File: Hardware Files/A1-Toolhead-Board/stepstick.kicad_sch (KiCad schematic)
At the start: 18 parts, among them J1 Motor_E, U1 TMC2209-LA

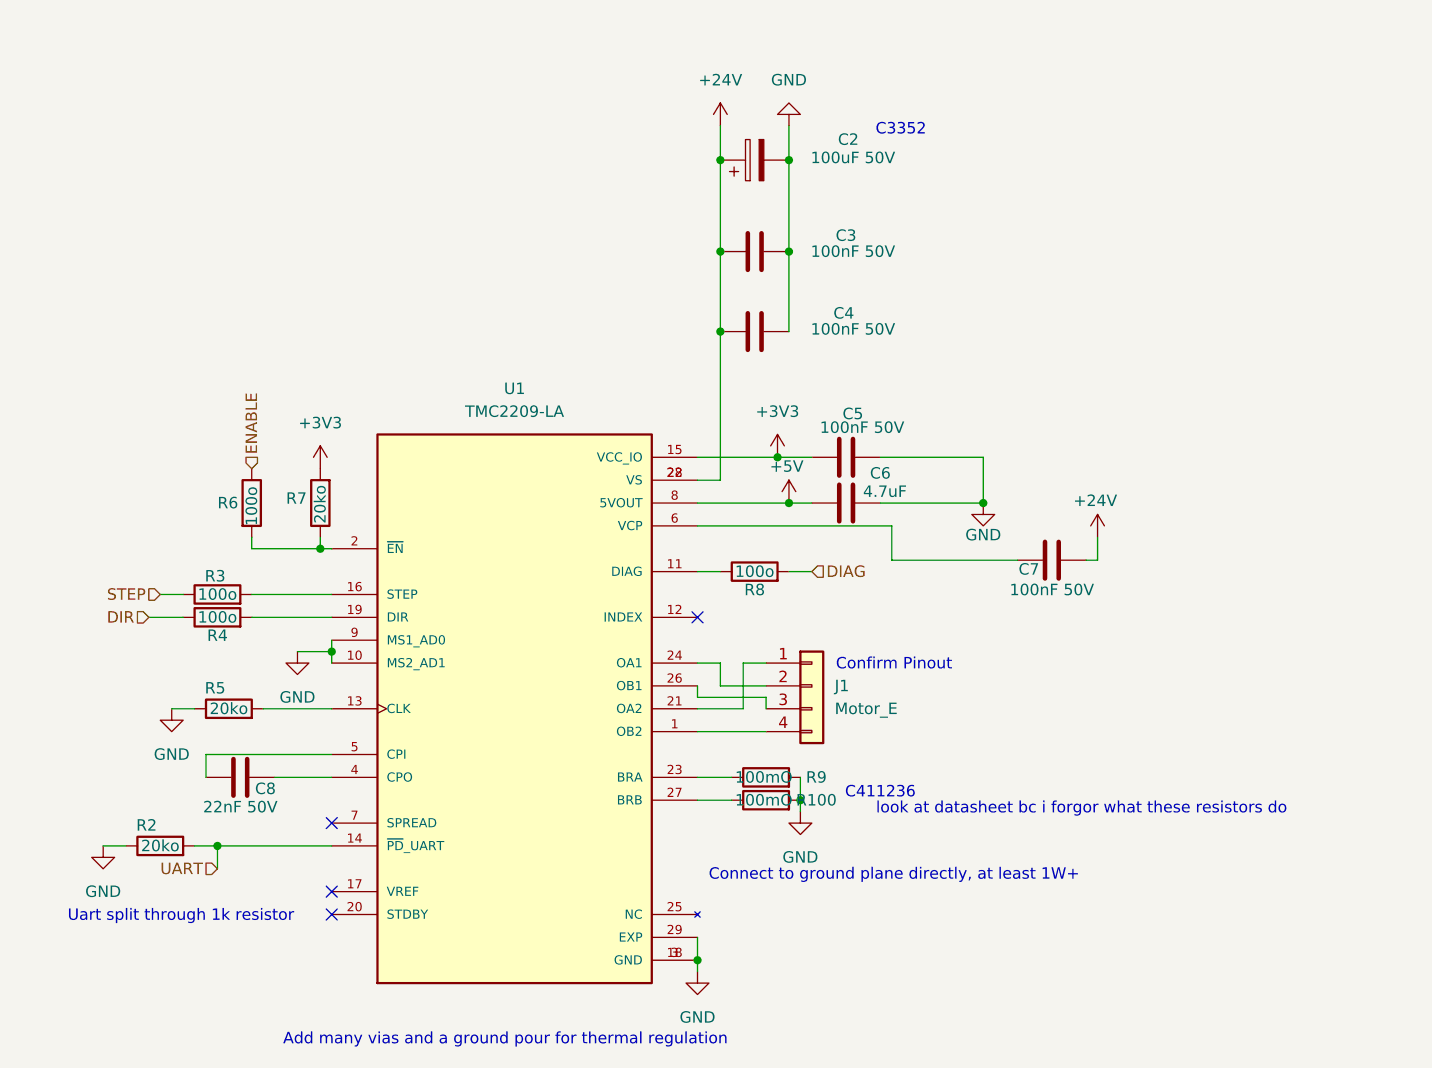
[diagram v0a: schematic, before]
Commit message: e
e
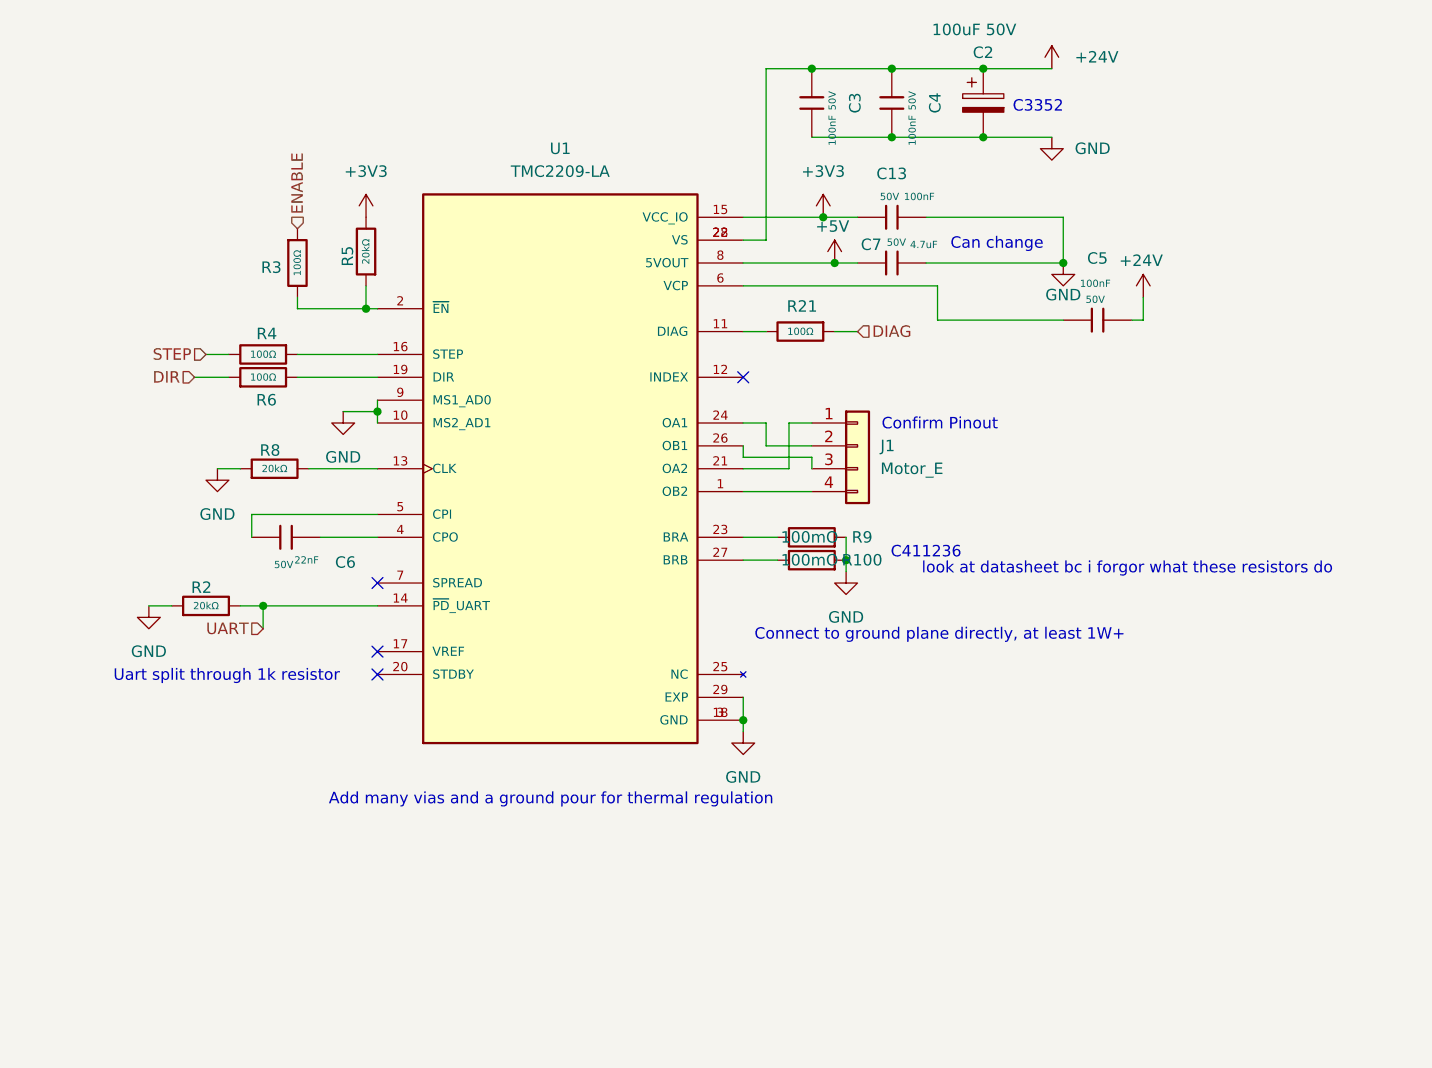
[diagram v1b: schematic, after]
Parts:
- removed C3, C4, C5, C7: 100nF 50V, Capacitor_SMD:C_0402_1005Metric, symbol Device:C
- removed C6: 4.7uF, Capacitor_SMD:C_0201_0603Metric, symbol Device:C
- removed C8: 22nF 50V, Capacitor_SMD:C_0402_1005Metric, symbol Device:C
- removed R2, R5, R7: 20ko, Resistor_SMD:R_0402_1005Metric, symbol Device:R
- removed R3, R4, R6, R8: 100o, Resistor_SMD:R_0402_1005Metric, symbol Device:R
- added C13, C3, C4, C5: 100nF, PCM_JLCPCB:C_0402, symbol PCM_JLCPCB-Capacitors:0402,100nF,(2)
- added C6: 22nF, PCM_JLCPCB:C_0402, symbol PCM_JLCPCB-Capacitors:0402,22nF
- added C7: 4.7uF, PCM_JLCPCB:C_1206, symbol PCM_JLCPCB-Capacitors:1206,4.7uF
- added R2, R5, R8: 20kΩ, PCM_JLCPCB:R_0402, symbol PCM_JLCPCB-Resistors:0402,20kΩ
- added R21, R3, R4, R6: 100Ω, PCM_JLCPCB:R_0402, symbol PCM_JLCPCB-Resistors:0402,100Ω
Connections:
- net +24V: now also C3.1, C4.1, C5.2
- net +3V3: now also C13.1, R5.2
- net +5V: now also C7.1
- net DIAG: now also R21.1
- net DIR: now also R6.1
- net ENABLE: now also R3.1
- net GND: now also C13.2, C3.2, C4.2, C7.2, R2.1, R8.1
- net STEP: now also R4.2
- net UART: now also R2.2
- net at U1.5 (CPI): now also C6.1
- net at U1.4 (CPO): now also C6.2
- net at U1.13 (CLK): now also R8.2
- net at U1.11 (DIAG): now also R21.2
- net at U1.16 (STEP): now also R4.1
- net at U1.19 (DIR): now also R6.2
- net at U1.2 (~{EN}): now also R3.2, R5.1
- net at U1.6 (VCP): now also C5.1
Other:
- note added: "Can change"
- moved on the sheet: C2, J1, R100, R9, U1

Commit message: e
e
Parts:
- U1: footprint Package_DFN_QFN:VQFN-28-1EP_5x5mm_P0.5mm_EP3.7x3.7mm_ThermalVias -> TMC2209-LA:TMC2209-LargerVias
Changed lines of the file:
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@@
 			)
 		)
-		(property "Footprint" "Package_DFN_QFN:VQFN-28-1EP_5x5mm_P0.5mm_EP3.7x3.7mm_ThermalVias"
+		(property "Footprint" "TMC2209-LA:TMC2209-LargerVias"
 			(at 69.85 63.5 0)
 			(hide yes)
